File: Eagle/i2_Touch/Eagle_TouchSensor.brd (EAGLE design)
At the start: 20 x 24.2 mm, 10 parts, among them U1 TTP223

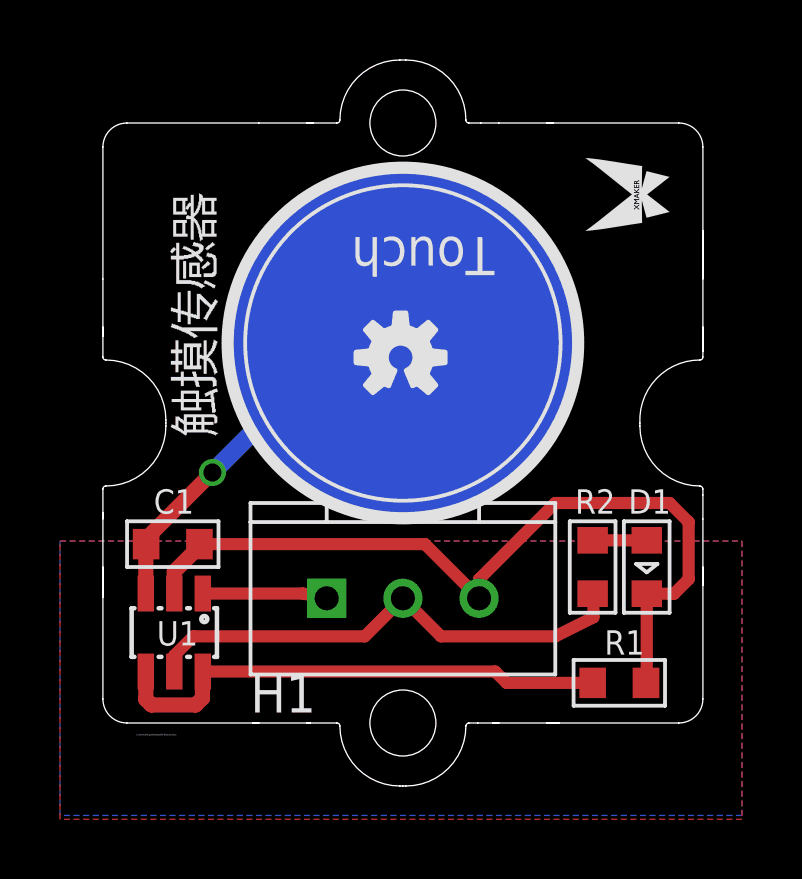
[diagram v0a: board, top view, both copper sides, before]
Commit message: chuange touch
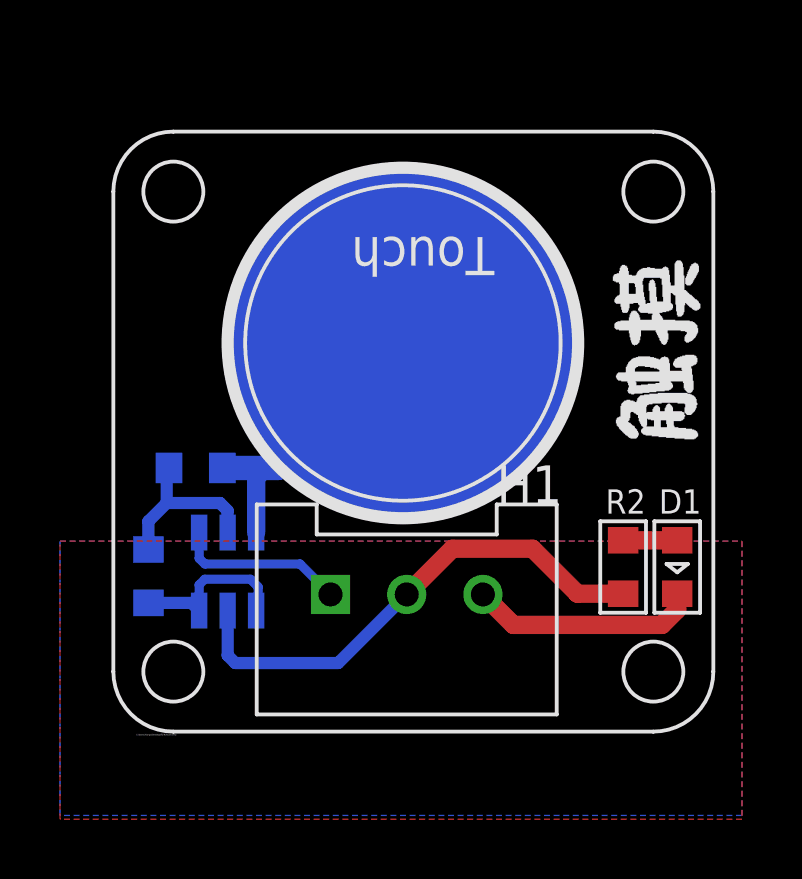
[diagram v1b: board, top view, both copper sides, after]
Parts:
- removed TWIG1: U1N, twig_template1:U1N
- removed U$2: (no value), SparkFun-Aesthetics:OSHW-LOGO-S
- added U$3: DIMENSION_2MM2MM, Xmaker:DIMENSION_2MM*2MM
- added U$4: NAME_TOUCH, Xmaker:NAME_TOUCH
- added U$5: OPENHARDWARE_2.5MM_TOP, Xmaker:OPENSOURCELOGO_2.5MM
- H1: value HEAD_LOCK -> HEAD_LOCK_3PIN_2; device HEAD_LOCK:HEAD_LOCK -> Xmaker:HEAD_LOCK_3PIN_2
- moved R1 16.1 mm to (0.41, 5.18), flipped to the bottom, turned to 90 degrees
- moved U$1 2.97 mm to (19.3, 13.2), flipped to the bottom, turned to 270 degrees
- moved U1 2.70 mm to (3.05, 5.33), flipped to the bottom
- moved H1 2.67 mm to (9.02, 4.57), turned to 90 degrees
- moved C1 2.65 mm to (1.98, 8.79), flipped to the bottom
- moved D1 1.02 mm to (18.0, 5.49)
- moved R2 1.02 mm to (16.2, 5.49)
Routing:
- net GND: track 27.9 -> 13.5 mm
- net N$2: track 17.0 -> 5.63 mm
- net IN: track 13.1 -> 10.0 mm, vias 1 -> 0
- net D1: track 4.15 -> 5.74 mm
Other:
- board outline removed
- board text removed: "GND"
- board text removed: "SIG"
- board text removed: "VCC"
